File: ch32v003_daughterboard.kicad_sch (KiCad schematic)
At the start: 10 parts, among them J1 Conn_02x05_Odd_Even, J2 Conn_01x03_Pin, J3 USB_B_Mini, P1 Header 7X2, P2 Header 7X2, U1 FT230XS

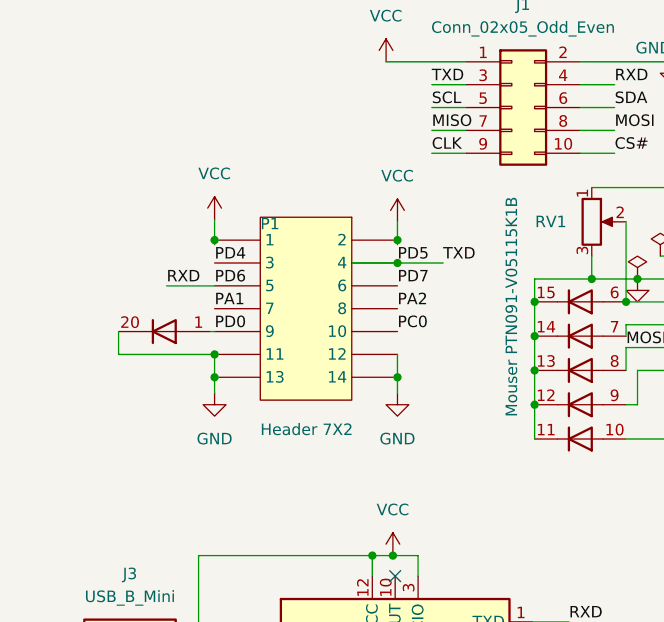
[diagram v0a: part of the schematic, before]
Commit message: add push button
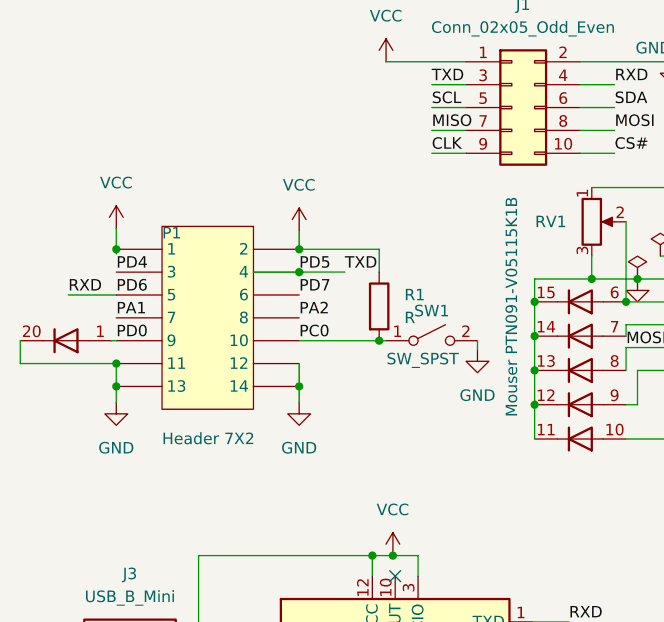
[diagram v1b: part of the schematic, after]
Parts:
- added R1: R, Resistor_SMD:R_0805_2012Metric_Pad1.20x1.40mm_HandSolder, symbol Device:R
- added SW1: SW_SPST, Button_Switch_SMD:SW_SPST_B3SL-1002P, symbol Switch:SW_SPST
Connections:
- net GND: now also SW1.2 (B)
- net PC0: now also R1.2, SW1.1 (A)
- net VCC: now also R1.1
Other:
- moved on the sheet: P1
